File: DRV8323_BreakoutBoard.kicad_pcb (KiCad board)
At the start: 4 copper layers, 40 x 40 mm, 33 parts, among them J2 Conn_01x09_Pin, J4 Conn_01x02_Pin, J6 Conn_01x09_Pin, Q1 30v_60a_Mosfet, Q2 30v_60a_Mosfet, Q3 30v_60a_Mosfet, Q4 30v_60a_Mosfet, Q5 30v_60a_Mosfet, Q6 30v_60a_Mosfet, U6 DRV8323S

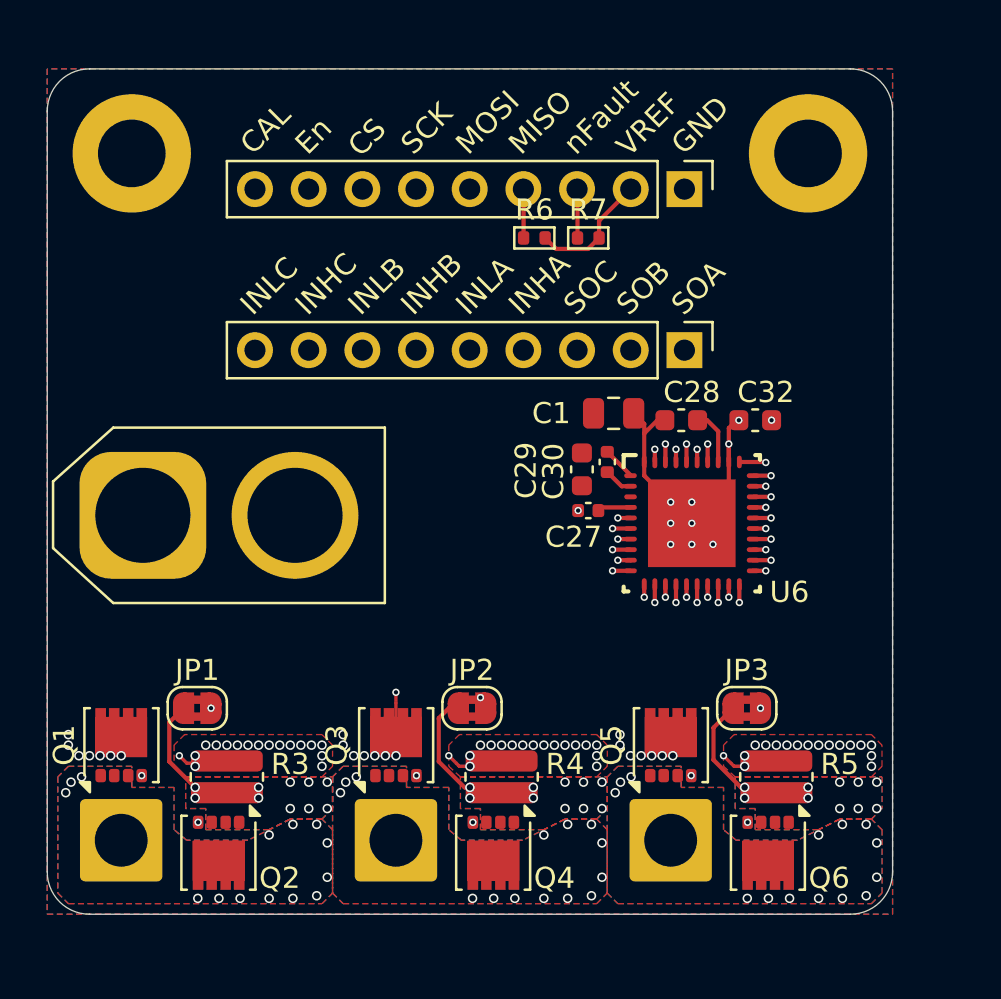
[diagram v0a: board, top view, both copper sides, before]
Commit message: V0
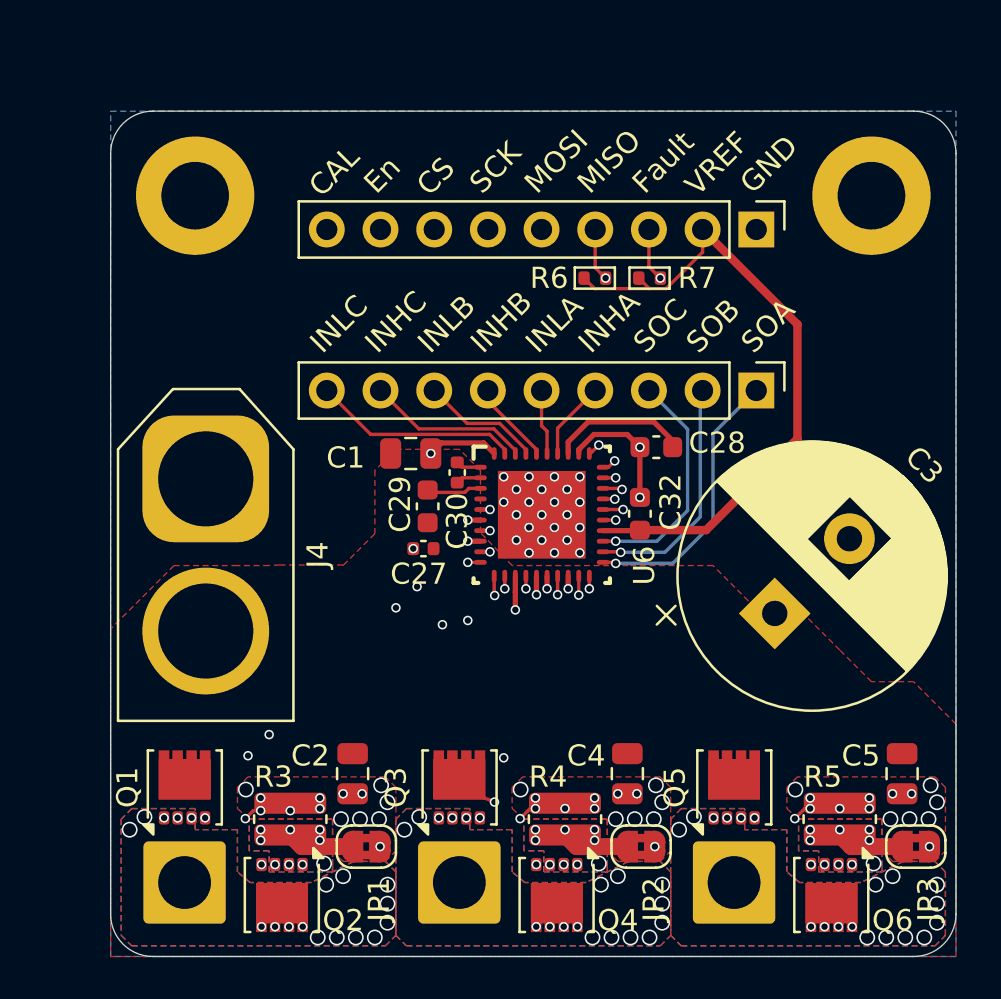
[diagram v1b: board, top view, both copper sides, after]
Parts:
- added C2: C_0805_10uF, Capacitor_SMD:C_0805_2012Metric, F.Cu at (62.5, 84.8)
- added C3: Cap_D12.5mm_1000uF, PCM_Capacitor_THT_AKL:CP_Radial_D12.5mm_P5.00mm, F.Cu at (82.4, 77.3)
- added C4: C_0805_10uF, Capacitor_SMD:C_0805_2012Metric, F.Cu at (75.5, 84.8)
- added C5: C_0805_10uF, Capacitor_SMD:C_0805_2012Metric, F.Cu at (88.5, 84.8)
- moved JP3 10.3 mm to (89.1, 88.3)
- moved JP1 10.3 mm to (63.1, 88.3)
- moved JP2 10.3 mm to (76.1, 88.3)
- moved C1 9.79 mm to (65.2, 69.7)
- moved C27 8.00 mm to (65.8, 74.2)
- moved C29 7.51 mm to (66.0, 72.2), turned to 90 degrees
- moved C30 7.12 mm to (67.4, 70.6)
- moved U6 7.11 mm to (71.4, 72.6)
- moved C32 7.03 mm to (76.0, 72.5), turned to 90 degrees
- moved NT1 6.57 mm to (68.9, 86.1), turned to 157.5 degrees
- moved NT3 4.27 mm to (70.5, 86.8), turned to -135 degrees
- moved NT4 4.27 mm to (83.5, 86.8), turned to -135 degrees
- moved NT2 4.08 mm to (57.5, 86.8), turned to -135 degrees
- moved J2 3.90 mm to (81.5, 59.1)
- moved J6 3.90 mm to (81.5, 66.7)
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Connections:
- J6 pad 1: SOA -> SOC
- J6 pad 3: SOC -> SOA
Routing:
- net SPC: track 6.84 -> 24.4 mm
- net CAL: track 34.8 -> 21.2 mm
- net INLB: track 18.4 -> 5.68 mm, vias 1 -> 0
- net INHC: track 20.3 -> 7.70 mm, vias 1 -> 0
- net INLC: track 22.2 -> 9.76 mm, vias 1 -> 0
- net INHB: track 16.2 -> 3.93 mm, vias 1 -> 0
- net INLA: track 14.3 -> 3.09 mm, vias 1 -> 0
- net Enable: track 33.0 -> 23.7 mm
- net GHA: track 29.0 -> 19.8 mm
- net CS: track 31.9 -> 22.9 mm
- net GLA: track 30.0 -> 21.2 mm
- net INHA: track 12.1 -> 3.72 mm, vias 1 -> 0
- net MA: track 31.8 -> 24.4 mm, vias 15 -> 19
- net VREF: track 38.4 -> 31.1 mm, vias 2 -> 0
- net GND: track 18.4 -> 11.3 mm, vias 58 -> 73
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- added copper zone on In2.Cu, net GND
- added copper zone on In4.Cu, net GND
- added copper zone on In3.Cu, net VIN
- removed copper zone on In2.Cu, net VIN
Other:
- copper layers 4 -> 6
- board text added: "Fault"
- board text added: "VIN"
- board text removed: "nFault"
